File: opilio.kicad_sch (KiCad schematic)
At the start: 23 parts, among them J1 Conn_01x04_Male, SW1 Reset, SW2 Boot, U1 STM32F103C8T6, Y1 YST310S 32.768KHz, Y2 TAXM8M4RFDCET2T

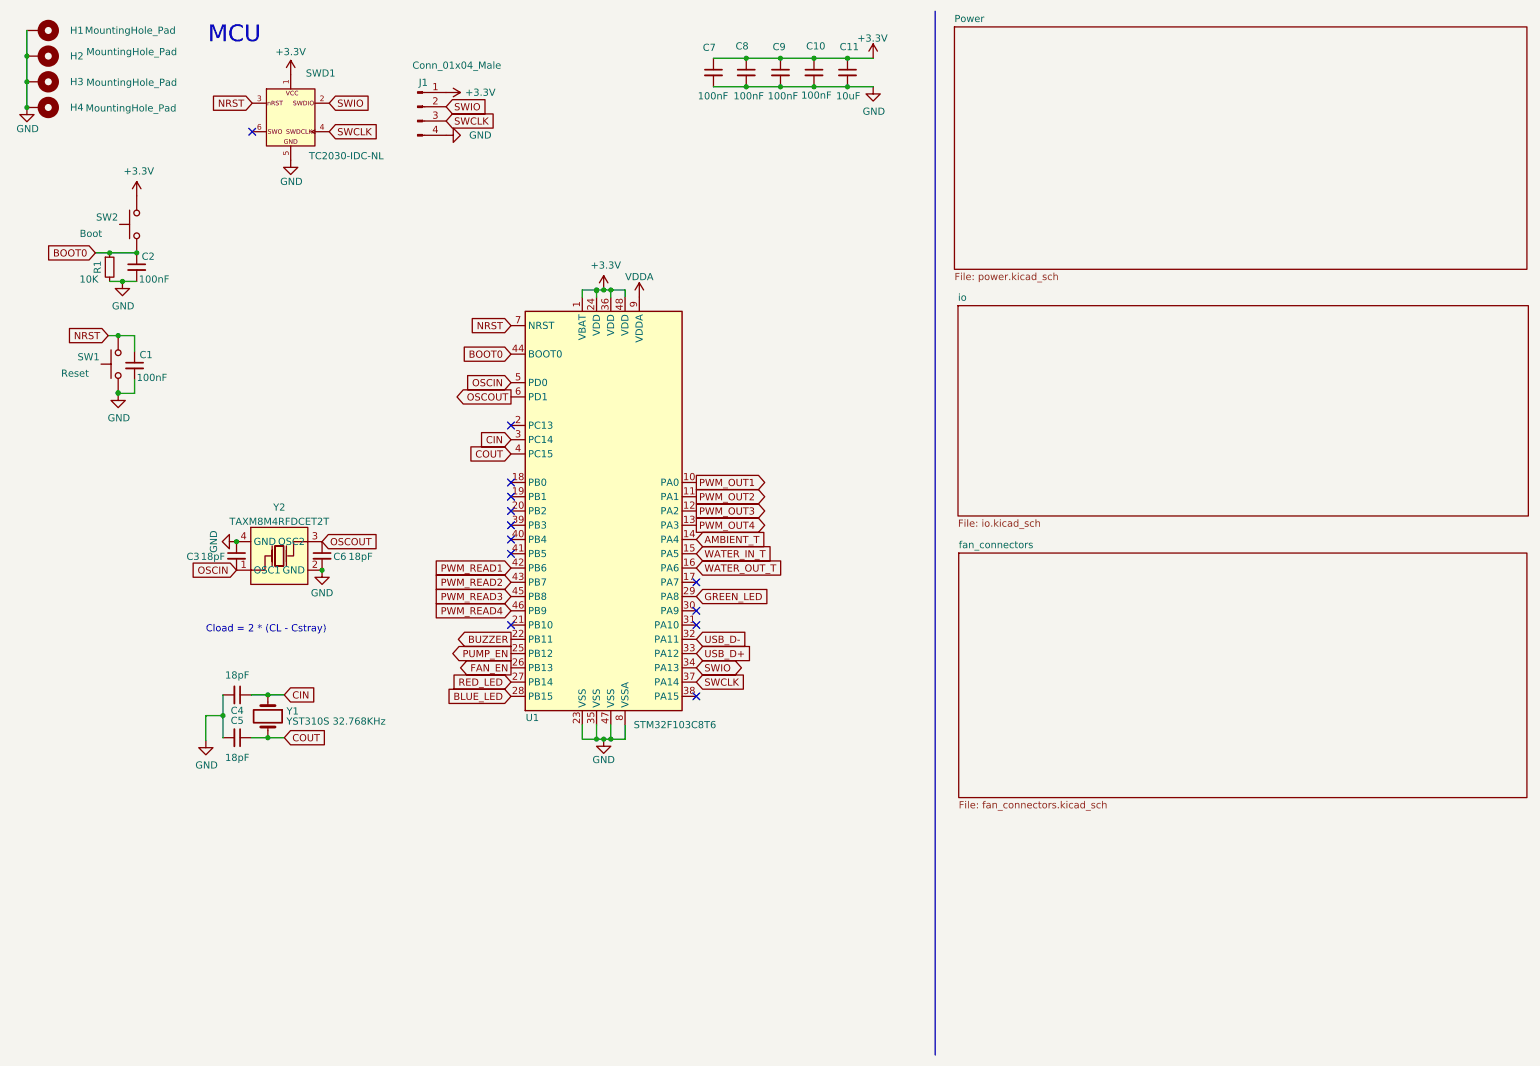
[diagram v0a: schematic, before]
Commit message: rev-7 ready
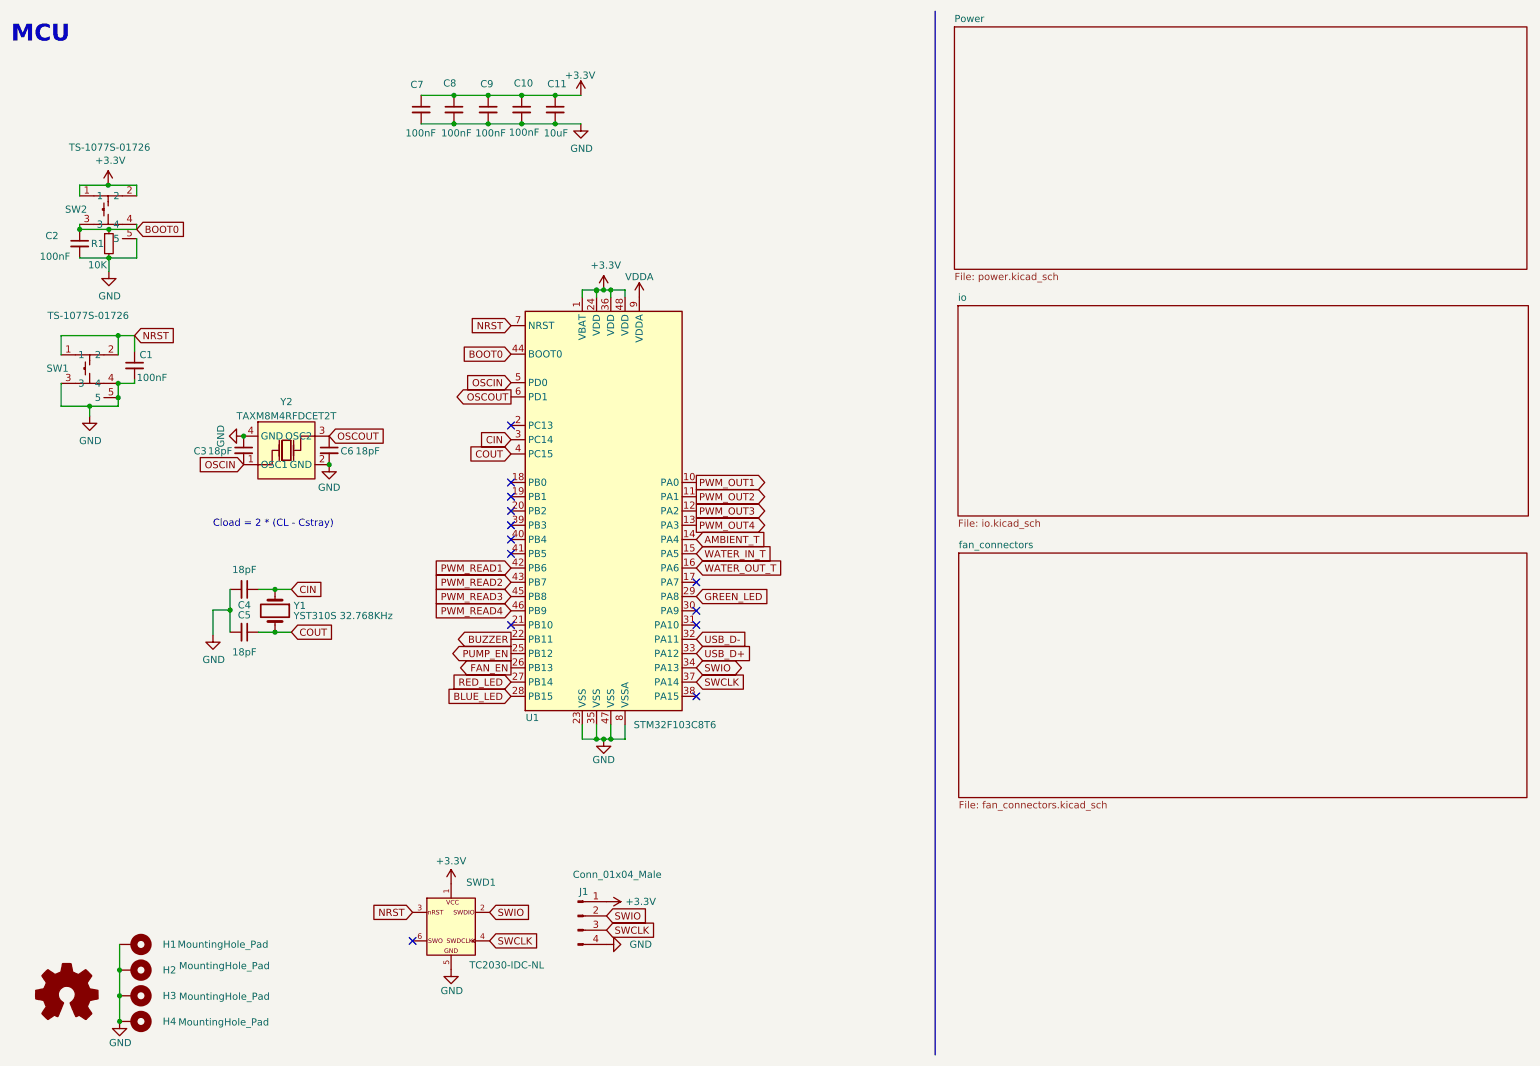
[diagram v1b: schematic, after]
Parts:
- removed SW1: Reset, easyeda2kicad:SW-SMD_L3.0-W2.5-P3.40-LS4.0-L, symbol Switch:SW_Push
- removed SW2: Boot, easyeda2kicad:SW-SMD_L3.0-W2.5-P3.40-LS4.0-L, symbol Switch:SW_Push
- added LOGO1: Logo_Open_Hardware_Small, Symbol:OSHW-Logo2_9.8x8mm_SilkScreen, symbol Graphic:Logo_Open_Hardware_Small
- added SW1, SW2: TS-1077S-01726, easyeda2kicad:KEY-SMD_4P-L3.1-W3.1-P2.00_TS-1077S-01726, symbol easyeda:TS-1077S-01726
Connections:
- net +3.3V: now also SW2.1, SW2.2
- net BOOT0: now also SW2.3, SW2.4
- net GND: now also SW1.3, SW1.4, SW1.5, SW2.5
- net NRST: now also SW1.1, SW1.2
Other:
- moved on the sheet: C10, C11, C2, C3, C4, C5, C6, C7, C8, C9, H1, H2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
